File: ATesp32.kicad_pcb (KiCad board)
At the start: 2 copper layers, 18 x 51.2 mm, 51 parts, among them J1 USB_C_Receptacle_USB2.0_16P, J2 JST PH, Q1 DMP2045U, SW1 SW_Push, SW2 SW_Push, U1 ESP32-S3, U2 ATmega32A-P, U3 MCP73831-2-OT, U4 AP2112K-3.3, U5 CP2102N-Axx-xQFN24, Y1 40 MHz

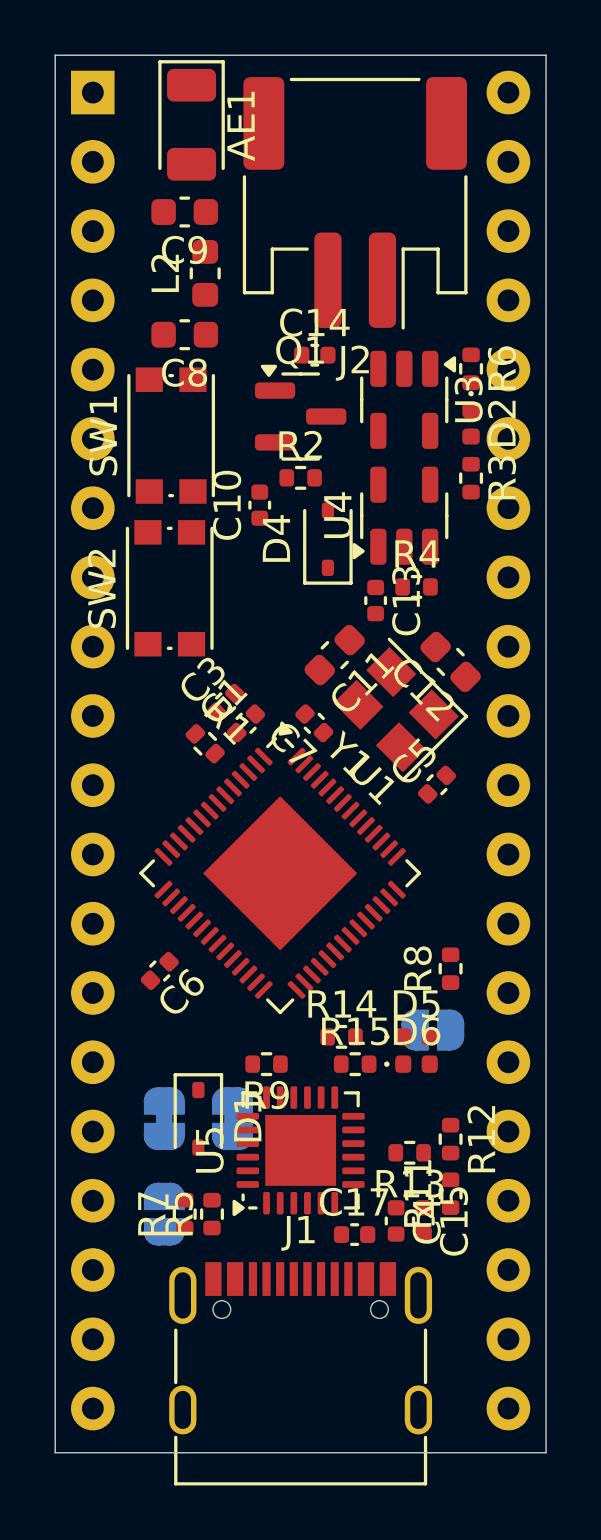
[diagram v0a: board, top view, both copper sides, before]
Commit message: Finished layout, need to fix silk
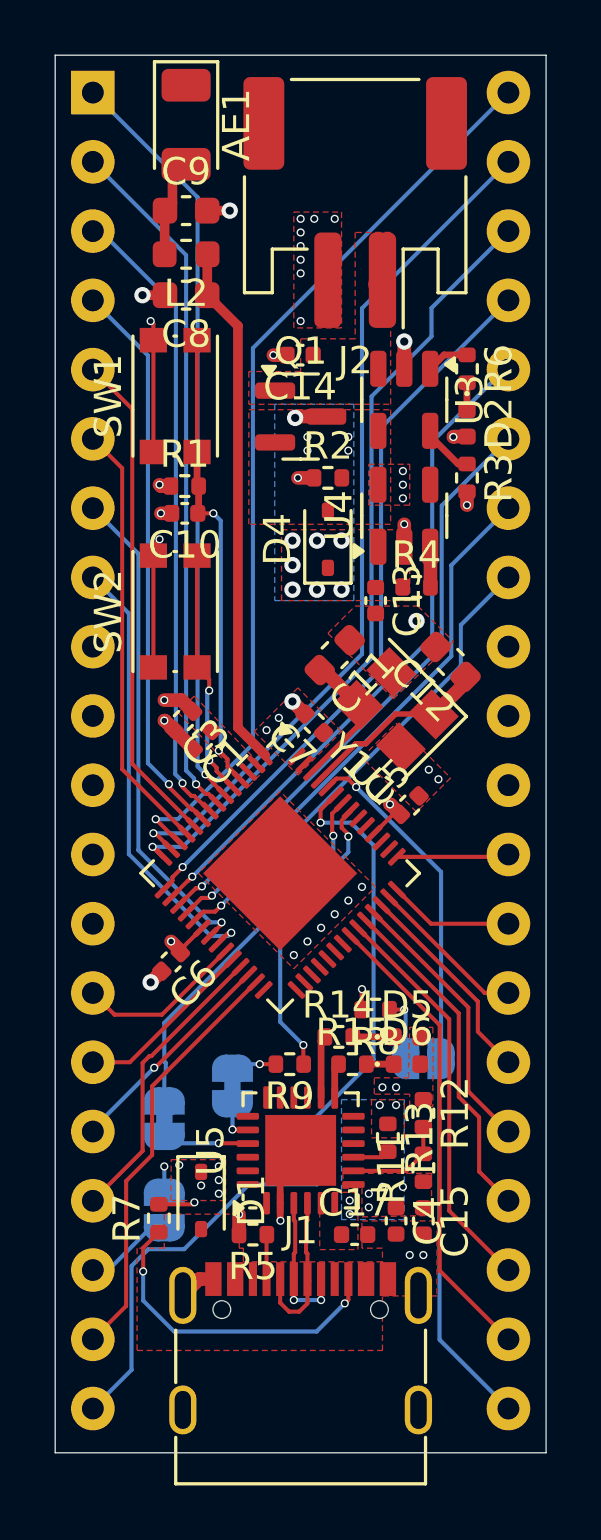
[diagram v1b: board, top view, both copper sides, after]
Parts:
- moved R1 9.48 mm to (79.8, 65.8), turned to 0 degrees
- moved R8 3.13 mm to (86.8, 85.0), turned to 180 degrees
- moved D1 3.00 mm to (80.3, 92.0)
- moved C10 2.77 mm to (79.8, 66.8), turned to 180 degrees
- moved C1 1.71 mm to (80.4, 75.1), turned to -135 degrees
- moved C3 1.68 mm to (79.7, 74.4), turned to -135 degrees
- moved R5 1.68 mm to (82.2, 93.2), turned to 180 degrees
- moved SW1 1.46 mm to (79.4, 62.5)
- moved C8 1.45 mm to (79.8, 58.8)
- moved R11 1.38 mm to (88.5, 90.8)
- moved R12 1.38 mm to (88.5, 88.8)
- moved C5 1.25 mm to (88.0, 77.5)
- moved JP8 1.20 mm to (81.5, 87.8)
- moved JP6 1.11 mm to (88.5, 86.8), turned to 180 degrees
- moved R2 1.00 mm to (85.0, 65.5)
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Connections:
- net Net-(U1-XTAL_N) renamed XTAL_N
- net Net-(U1-XTAL_P) renamed XTAL_P
- net PD2_P renamed D_P
- net PD3_N renamed D_N
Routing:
- net PA0: track 0.00 -> 33.7 mm, vias 0 -> 1
- net PA1: track 0.00 -> 31.5 mm, vias 0 -> 1
- net PD6: track 0.00 -> 30.7 mm, vias 0 -> 1
- net PA2: track 0.00 -> 29.2 mm, vias 0 -> 1
- net PB0: track 0.00 -> 27.8 mm, vias 0 -> 1
- net PA3: track 0.00 -> 26.9 mm, vias 0 -> 1
- net Net-(JP4-B): track 0.00 -> 26.7 mm, vias 0 -> 3
- net PD7: track 0.00 -> 25.9 mm, vias 0 -> 1
- net PB1: track 0.00 -> 25.5 mm, vias 0 -> 1
- net GND: track 0.00 -> 25.4 mm, vias 0 -> 39
- net PA4: track 0.00 -> 24.6 mm, vias 0 -> 1
- net PB2: track 0.00 -> 23.3 mm, vias 0 -> 1
- net PA5: track 0.00 -> 22.2 mm, vias 0 -> 1
- net PB3: track 0.00 -> 20.7 mm, vias 0 -> 1
- net PA6: track 0.00 -> 19.9 mm, vias 0 -> 1
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- added copper zone on F.Cu, net +3V3
- added copper zone on In2.Cu, net +3V3
- added copper zone on F.Cu, net +5V
- added copper zone on In2.Cu, net +5V
- added copper zone on F.Cu, net +BATT
- added copper zone on F.Cu, net GND
- added copper zone on In1.Cu, net GND
- added copper zone on F.Cu, net Net-(D1-A)
- added copper zone on B.Cu, net Net-(D4-K)
- added copper zone on F.Cu, net Net-(D4-K)
- added copper zone on B.Cu, net Net-(U5-VDD)
- added copper zone on F.Cu, net Net-(U5-VDD)
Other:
- copper layers 2 -> 4
